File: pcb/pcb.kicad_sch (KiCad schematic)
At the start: 10 parts

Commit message: Footprins for electronics
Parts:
- BATTERY_1: footprint SelfBalancingRobot:Untitled -> SelfBalancingRobot:Battery_Connection_01x02
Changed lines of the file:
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@@
 			)
 		)
-		(property "Footprint" "SelfBalancingRobot:Untitled"
+		(property "Footprint" "SelfBalancingRobot:Battery_Connection_01x02"
 			(at 109.22 143.51 0)
 			(hide yes)

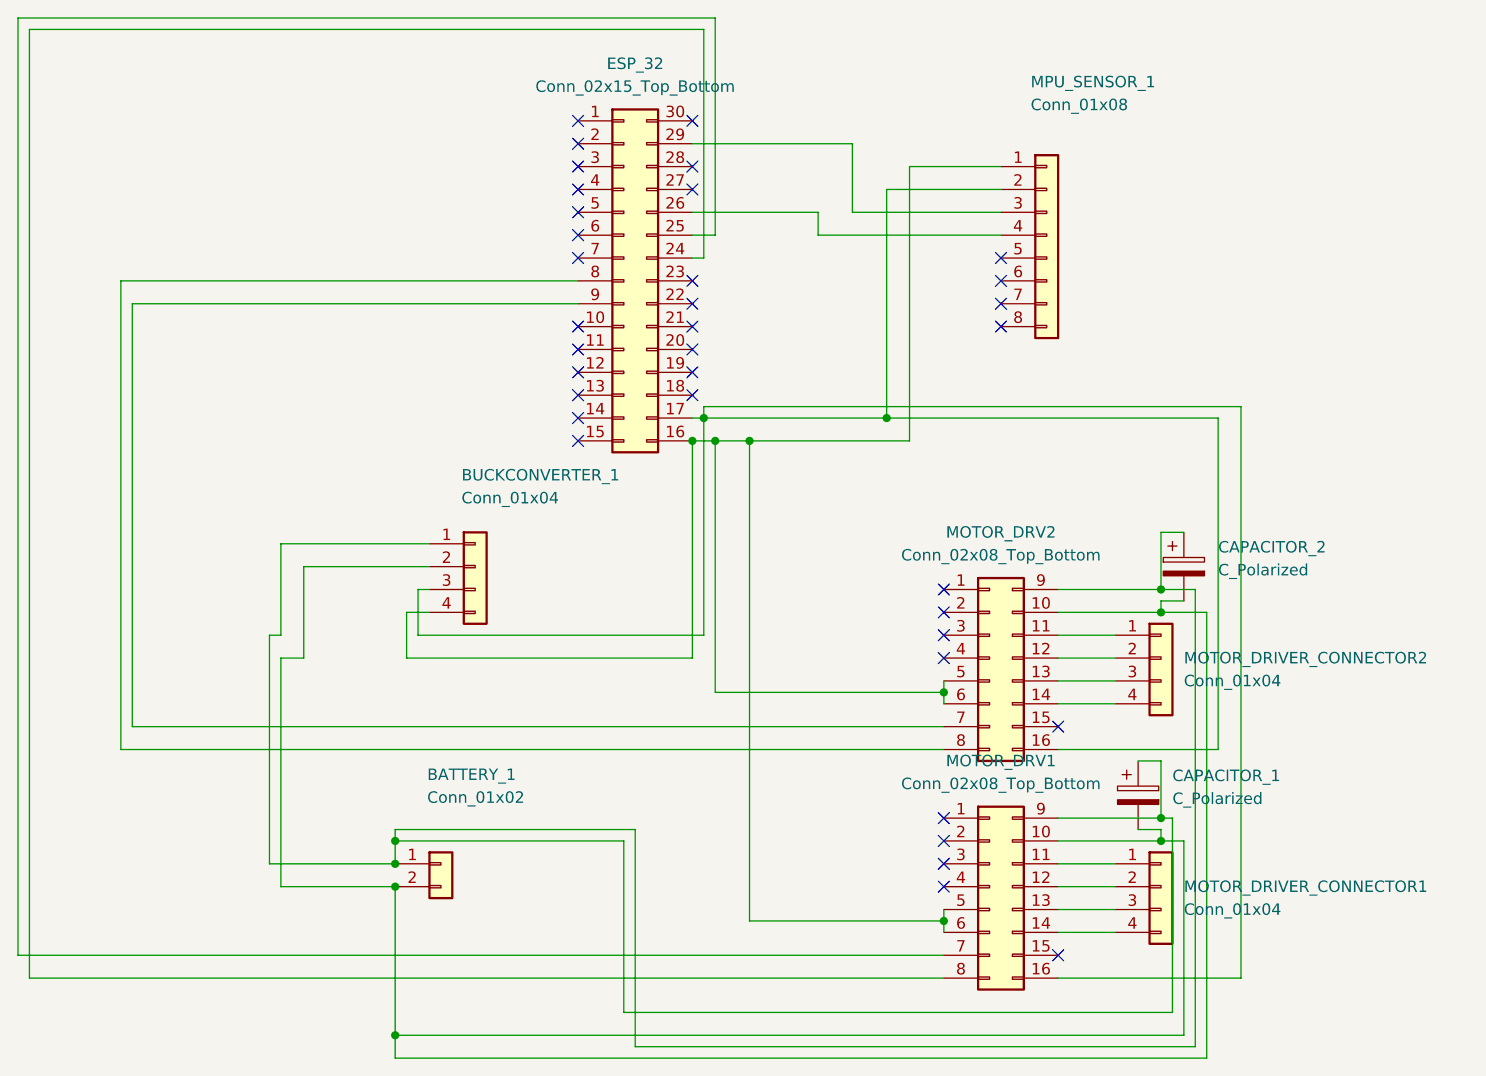
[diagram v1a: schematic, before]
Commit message: Finalized PCB version 1
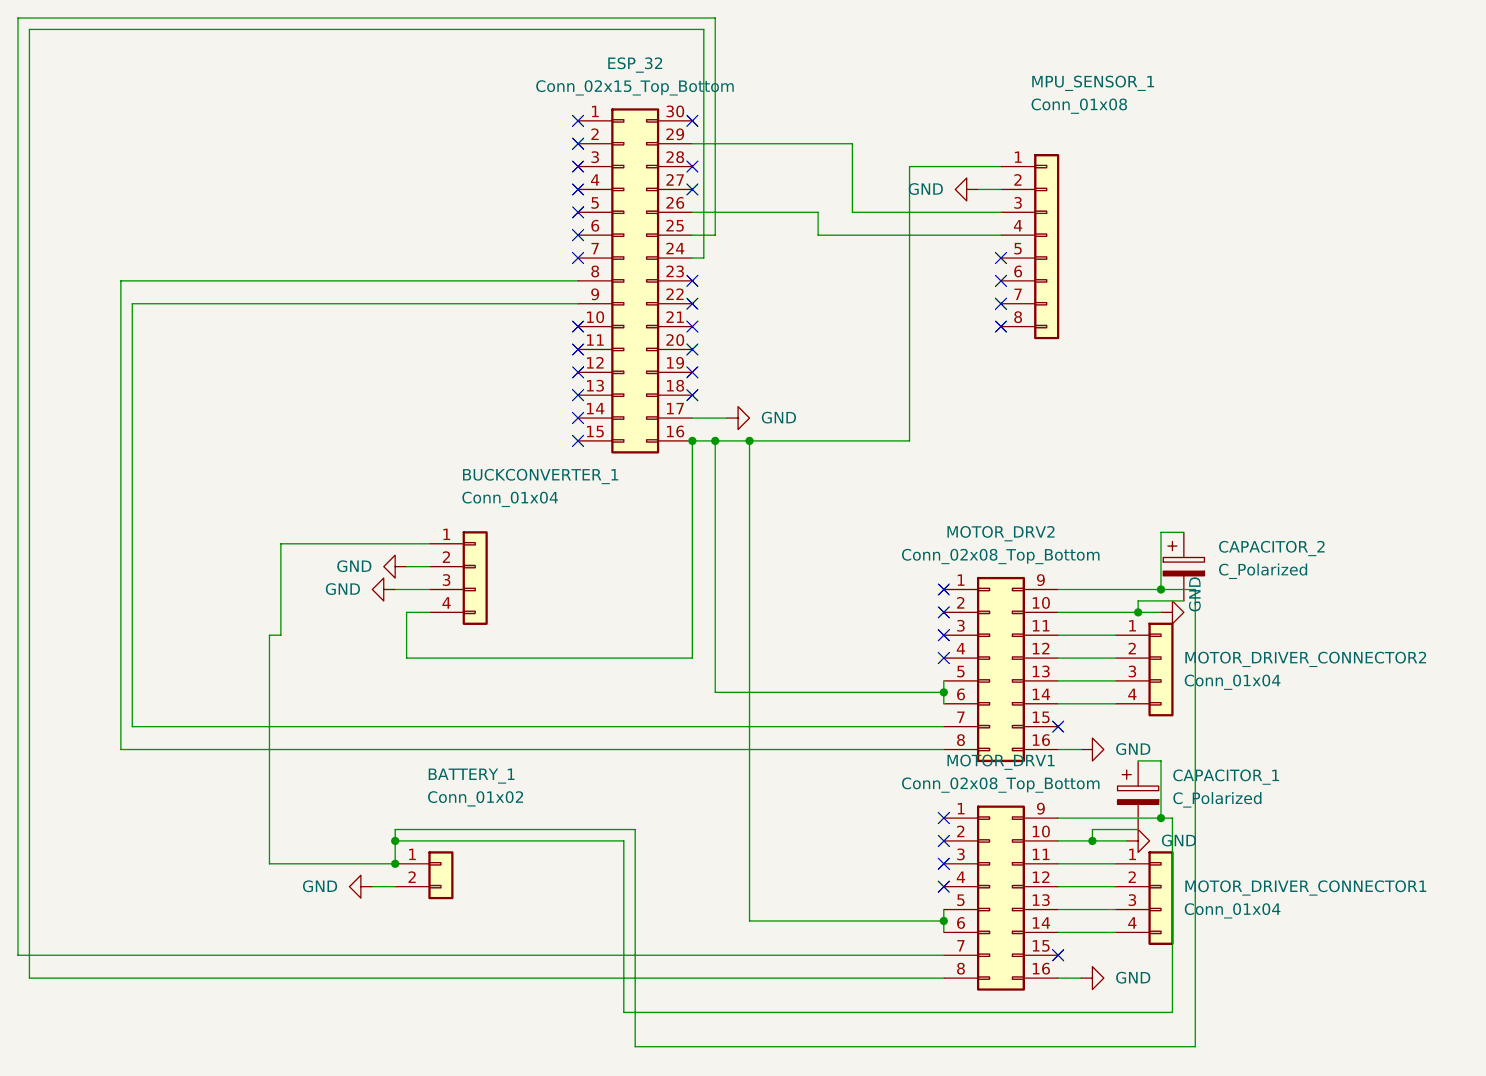
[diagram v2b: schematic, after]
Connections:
- net GND: now reaches BUCKCONVERTER_1.3 (GND), ESP_32.17 (GND), MOTOR_DRV1.16 (Pin_16), MOTOR_DRV2.16 (Pin_16), MPU_SENSOR_1.2 (GND)
- net GND: now also BATTERY_1.2 (GND), BUCKCONVERTER_1.2 (Pin_2), CAPACITOR_1.2, CAPACITOR_2.2, MOTOR_DRV1.10 (GND), MOTOR_DRV2.10 (GND)
